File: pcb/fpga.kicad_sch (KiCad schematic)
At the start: 27 parts

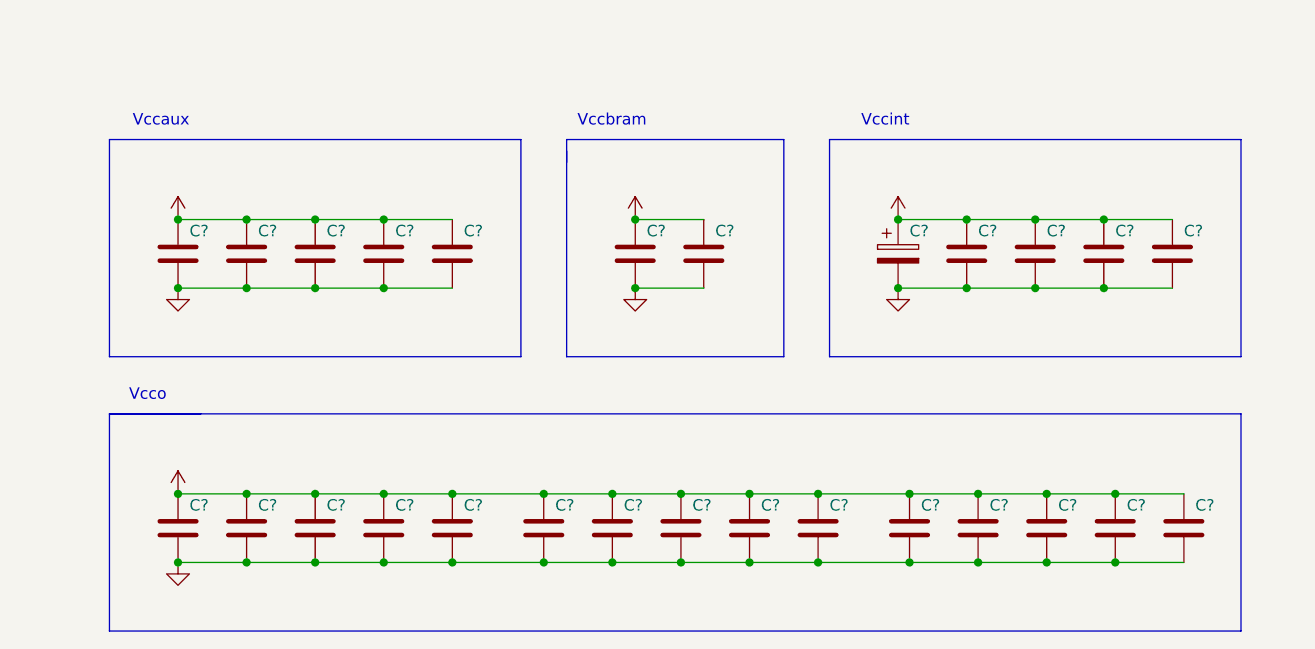
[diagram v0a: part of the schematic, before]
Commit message: kicad said I needed to save
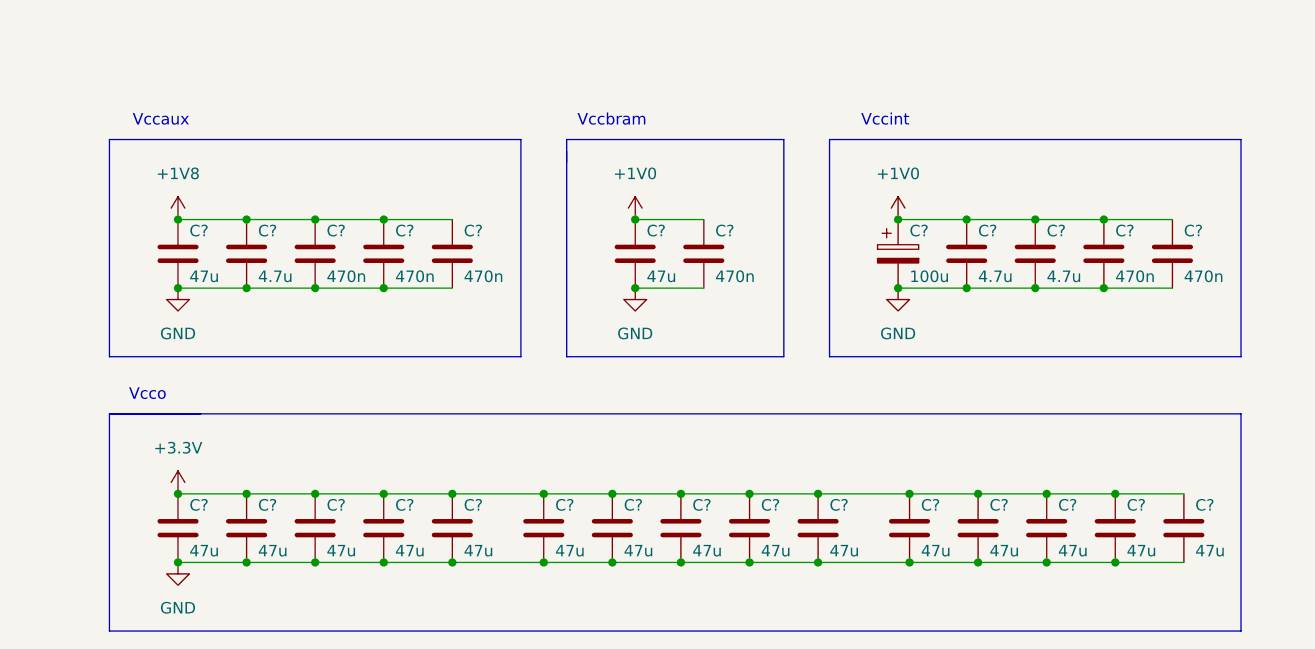
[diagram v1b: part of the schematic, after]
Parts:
- C? (x17): value (none) -> 47u; footprint (none) -> Capacitor_SMD:C_0805_2012Metric_Pad1.18x1.45mm_HandSolder
- C? (x6): value (none) -> 470n; footprint (none) -> Capacitor_SMD:C_0805_2012Metric_Pad1.18x1.45mm_HandSolder
- C? (x3): value (none) -> 4.7u; footprint (none) -> Capacitor_SMD:C_0805_2012Metric_Pad1.18x1.45mm_HandSolder
- C?: value (none) -> 100u

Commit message: add flash memory component for fpga
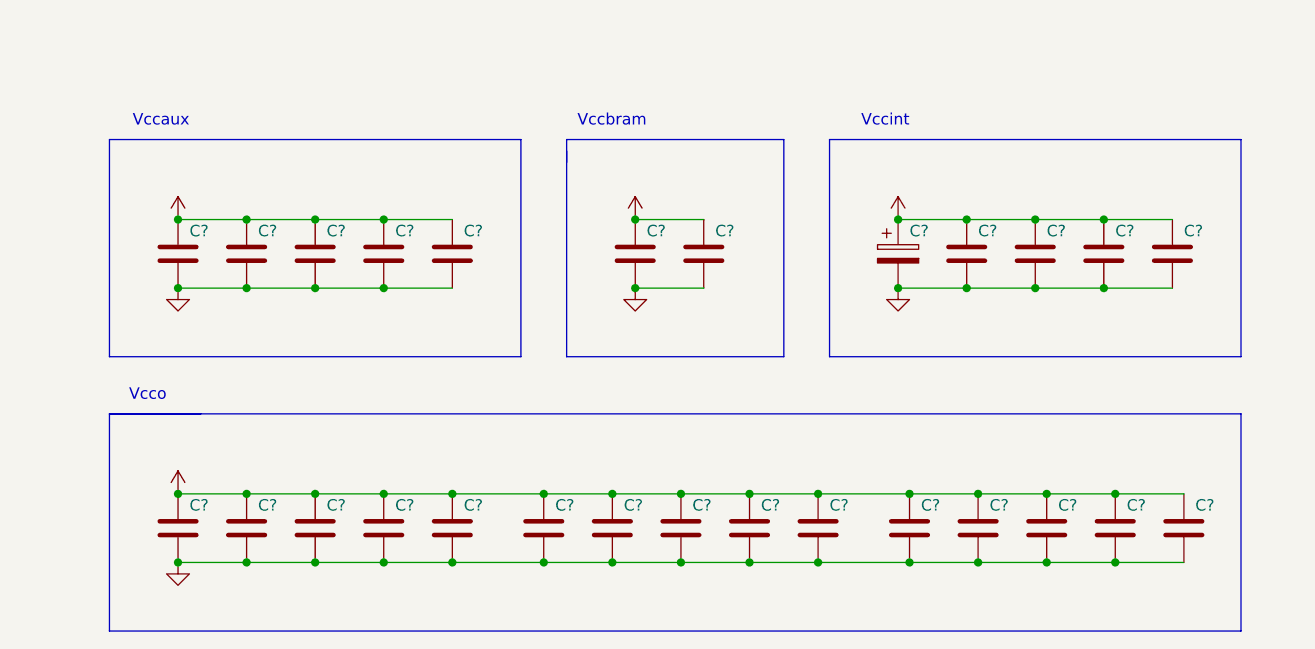
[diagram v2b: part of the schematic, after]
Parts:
- C? (x17): value 47u -> (none); footprint Capacitor_SMD:C_0805_2012Metric_Pad1.18x1.45mm_HandSolder -> (none)
- C? (x6): value 470n -> (none); footprint Capacitor_SMD:C_0805_2012Metric_Pad1.18x1.45mm_HandSolder -> (none)
- C? (x3): value 4.7u -> (none); footprint Capacitor_SMD:C_0805_2012Metric_Pad1.18x1.45mm_HandSolder -> (none)
- C?: value 100u -> (none)
